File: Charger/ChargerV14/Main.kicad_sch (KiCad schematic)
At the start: 23 parts, among them J1 TX_Coil, J6 Coil B, J8 USB_C_Receptacle_USB2.0, J9 Coil A, U2 XKT335, U3 XKT001

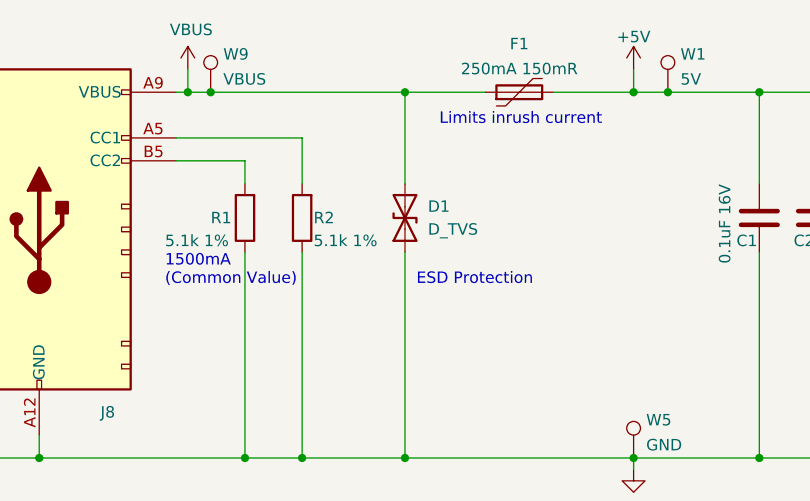
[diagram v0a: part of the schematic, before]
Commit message: Single Charger V14
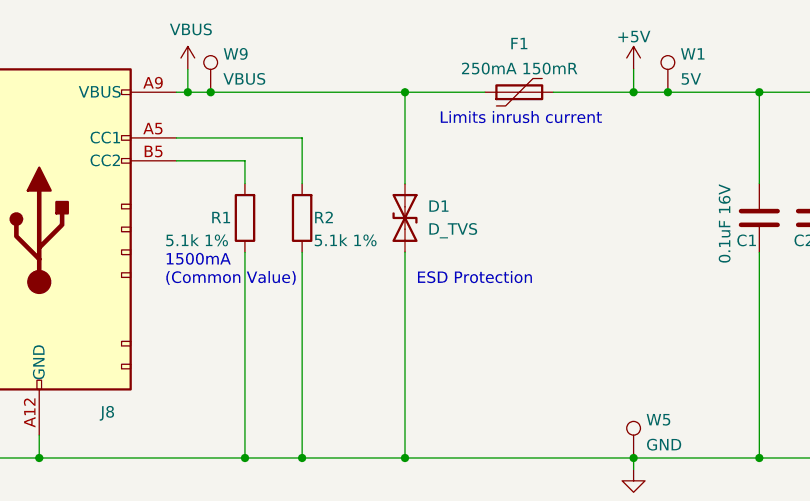
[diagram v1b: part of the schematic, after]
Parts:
- D1: footprint Diode_SMD:D_0402_1005Metric -> Pixels-dice:DFN
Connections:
- net GND: now also D1.2 (A2); no longer D1.1 (A1)
- net VBUS: now also D1.1 (A1); no longer D1.2 (A2)
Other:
- moved on the sheet: D1
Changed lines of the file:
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@@
     (pin "1")
   )
-  (symbol (lib_id "Device:D_TVS") (at 85.09 91.44 90) (unit 1)
+  (symbol (lib_id "Device:D_TVS") (at 85.09 91.44 270) (unit 1)
     (in_bom yes) (on_board yes) (fields_autoplaced)
     (property "Reference" "D1" (id 0) (at 87.63 90.1699 90)
-      (effects (font (size 1.27 1.27)) (justify right))
+      (effects (font (size 1.27 1.27)) (justify left))
     )
     (property "Value" "D_TVS" (id 1) (at 87.63 92.7099 90)
-      (effects (font (size 1.27 1.27)) (justify right))
+      (effects (font (size 1.27 1.27)) (justify left))
     )
-    (property "Footprint" "Diode_SMD:D_0402_1005Metric" (id 2) (at 85.09 91.44 0)
+    (property "Footprint" "Pixels-dice:DFN" (id 2) (at 85.09 91.44 0)
       (effects (font (size 1.27 1.27)) hide)
     )
@@
     )
     (path "/a3639dc2-2d4b-4f18-85bb-e7c6acafb9c8"
-      (reference "D1") (unit 1) (value "D_TVS") (footprint "Diode_SMD:D_0402_1005Metric")
+      (reference "D1") (unit 1) (value "D_TVS") (footprint "Pixels-dice:DFN")
     )
     (path "/fd0dfb1f-92bb-49bf-83f6-a5e3c0effca1"
